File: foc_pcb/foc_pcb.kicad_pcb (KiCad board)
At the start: 2 copper layers, 114.3 x 128.3 mm, 70 parts, among them IC1 AS5600-ASOT, J1 Conn_01x03, J10 Conn_02x03_Top_Bottom, J11 Conn_01x03, J12 10118193-0001LF, J2 Conn_01x03, J3 Conn_01x03, J4 Conn_01x04, J5 XT60PW-M, J6 XT60PW-M, J7 Conn_01x02, J8 Conn_01x02, J9 Conn_01x02, SW1 SW_Push, U1 DRV8313PWPR, U2 ATMEGA328P-AU, U3 BSS138-7-F, U4 BSS138-7-F, U5 CH340C, Y1 ABM3-16MHZ

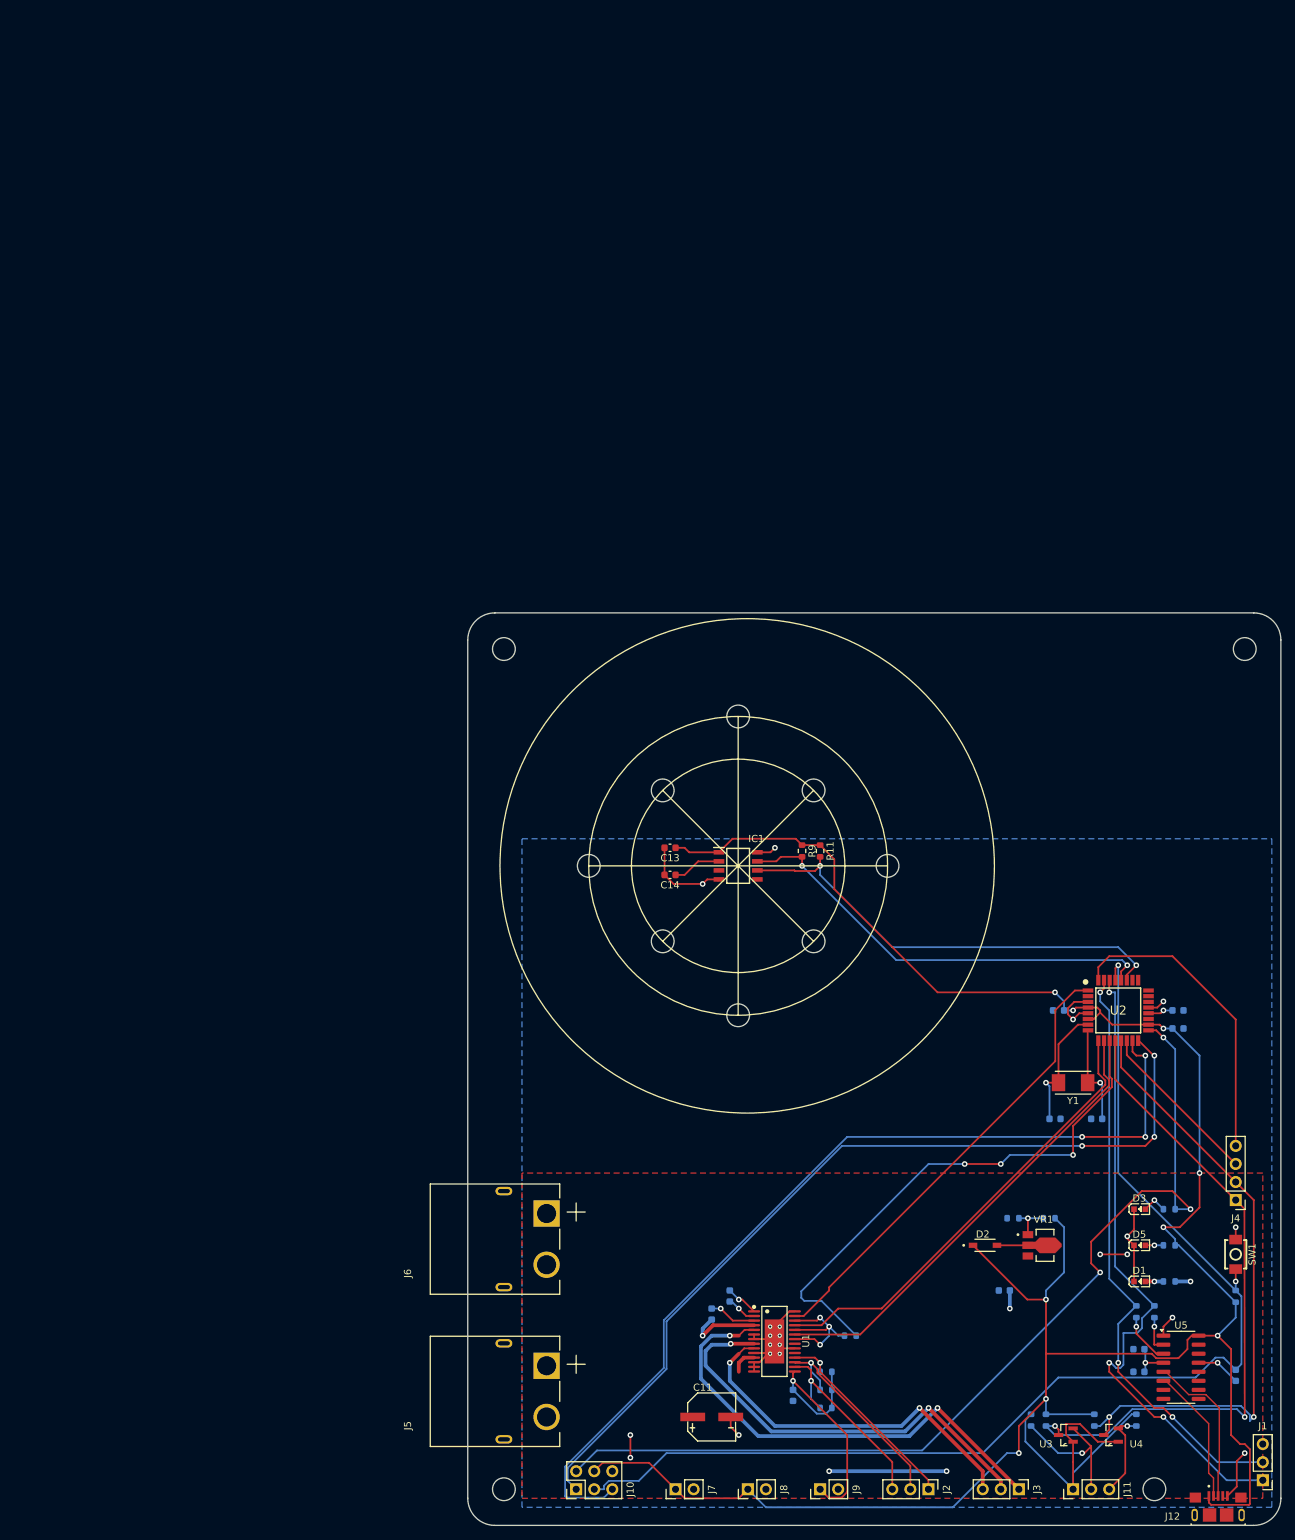
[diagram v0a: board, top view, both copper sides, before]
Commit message: V2 redesign done, needs review
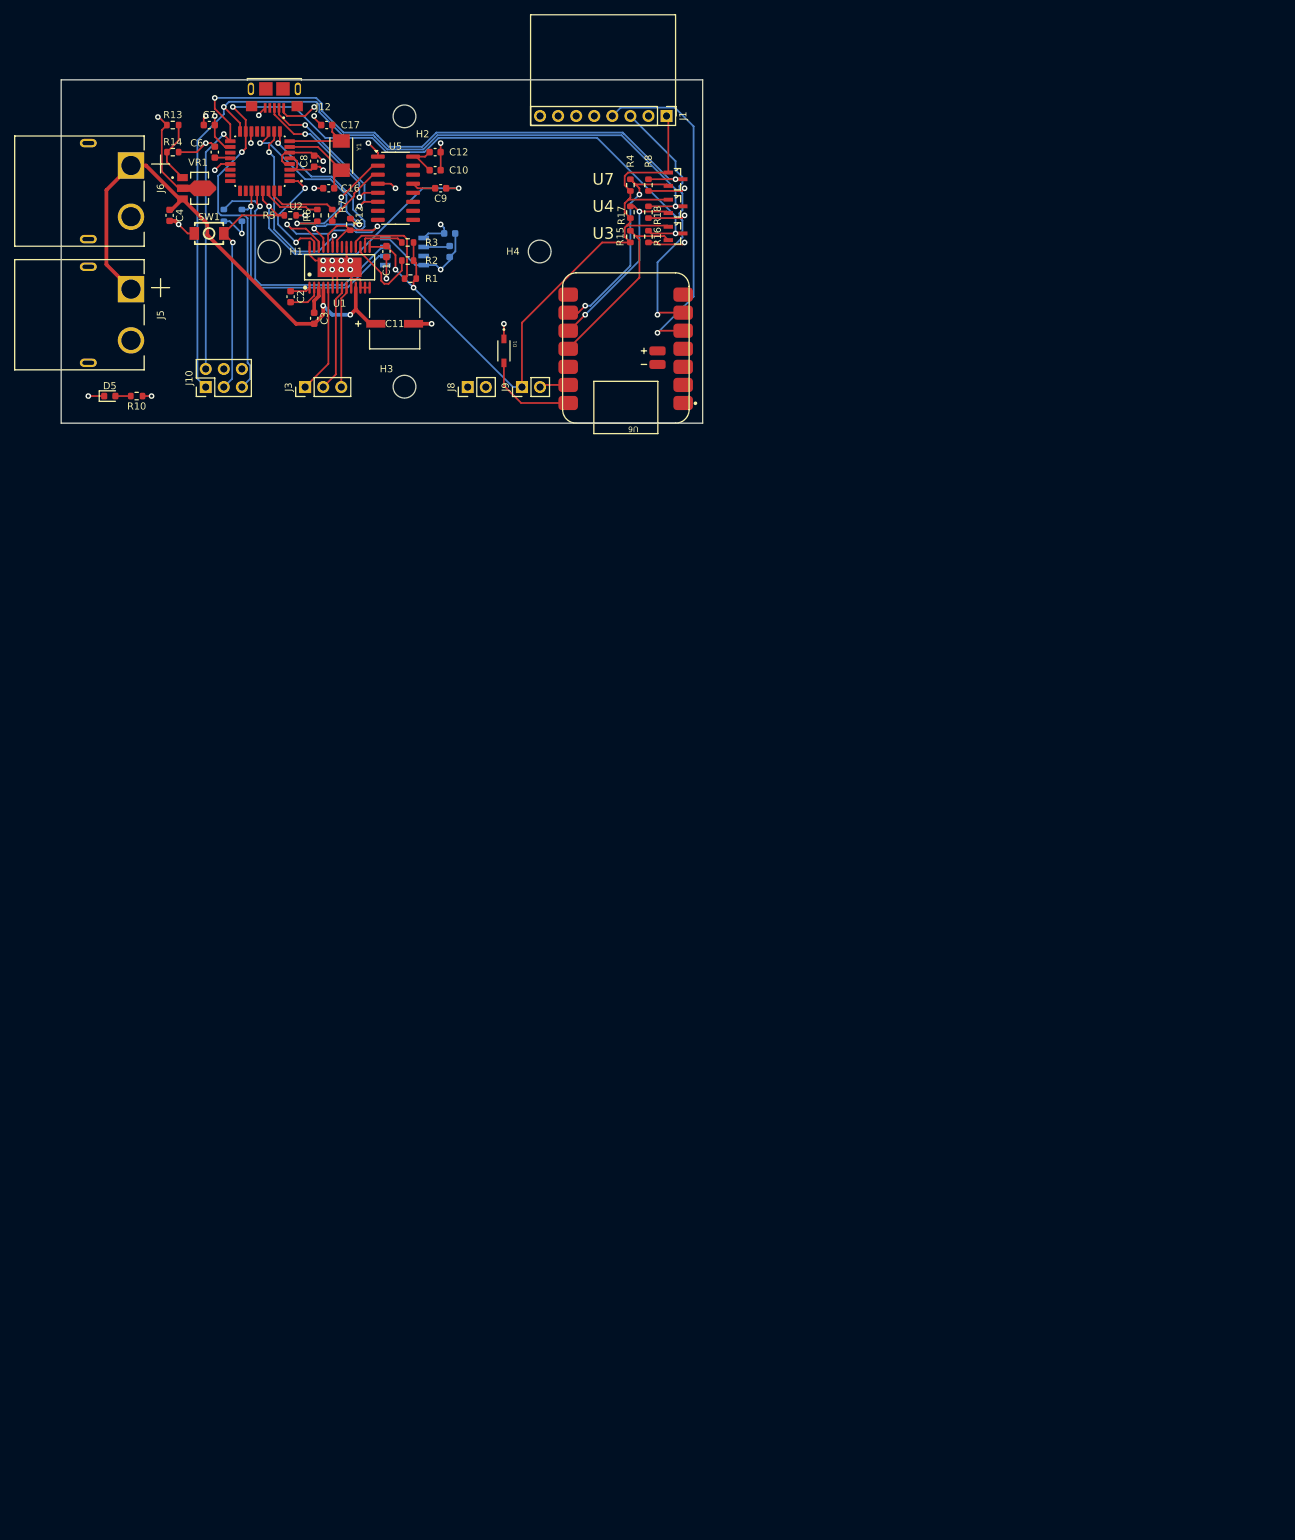
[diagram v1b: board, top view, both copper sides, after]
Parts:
- removed D2: 1N5819HW-7-F, 1N5819HW-7-F:SOD3715X145N
- removed D3: LED, KT-0603R:LED0603-RD
- removed H10, H11, H12, H9: boardMount, MountingHole:MountingHole_3.2mm_M3
- removed H5, H6, H7, H8: motorMount, MountingHole:MountingHole_3.2mm_M3
- removed J11, J2: Conn_01x03, Connector_PinHeader_2.54mm:PinHeader_1x03_P2.54mm_Vertical
- removed J4: Conn_01x04, Connector_PinHeader_2.54mm:PinHeader_1x04_P2.54mm_Vertical
- removed J7: Conn_01x02, Connector_PinHeader_2.54mm:PinHeader_1x02_P2.54mm_Vertical
- added U6: ~, XIAO-ESP32S3:MOUDLE14P-SMD-2.54-21X17.8MM, F.Cu at (287.7, 126.4)
- added U7: BSS138-7-F, BSS138-7-F:SOT95P240X110-3N, F.Cu at (285.8, 113.0)
- C1, C10, C12, C16, C17, C2, C3, C4, C6, C7, C8, C9, R1, R10, R12, R13, R14, R15, R16, R17, R18, R2, R3, R5, R6, R7: moved to F.Cu
- C11: value VT1V101M-CRE77 -> UWT1V101MCL1GS; footprint VT1V101M-CRE77:CAP-SMD_BD6.3-L6.6-W6.6-FD -> UWT1V101MCL1GS:PCAP_6.3x7.7-ELECT_NCA-L
- C13, C14, IC1, R11, R9: moved to B.Cu
- D1: value 19-213/Y2C-CQ2R2L/3T(CY) -> 1N5819HW-7-F; footprint simpleFOC_led:LED0603-RD-YELLOW -> 1N5819HW-7-F:SOD3715X145N
- D5: footprint KT-0603R:LED0603-RD -> LED_SMD:LED_0603_1608Metric
- J1: value Conn_01x03 -> MPU6050; footprint Connector_PinHeader_2.54mm:PinHeader_1x03_P2.54mm_Vertical -> Connector_PinHeader_2.54mm:PinHeader_1x08_P2.54mm_Vertical
- R4, R8: value 1k -> 10k; moved to F.Cu
- U2: footprint ATMEGA328P-AU-NEW:QFP80P900X900X120-32N -> ATMEGA328P-AU:QFP80P900X900X120-32N
- moved J12 240.4 mm to (229.4, 100.3), turned to 180 degrees
- moved J1 209.3 mm to (284.5, 104.1), turned to -90 degrees
- moved SW1 203.5 mm to (220.2, 120.7), turned to 0 degrees
- moved R5 201.9 mm to (231.6, 118.1), turned to 0 degrees
- moved C9 200.8 mm to (252.7, 114.3), turned to 180 degrees
- moved U5 199.2 mm to (246.4, 114.3)
- moved C12 197.9 mm to (252.0, 109.2), turned to 180 degrees
- moved R13 197.0 mm to (215.1, 105.4), turned to 0 degrees
- moved R6 193.9 mm to (235.4, 118.1)
- moved C10 193.0 mm to (252.0, 111.8), turned to 0 degrees
- moved C4 191.3 mm to (214.6, 118.1), turned to -90 degrees
- moved R7 191.1 mm to (237.5, 118.1)
- moved R14 190.8 mm to (215.1, 109.2), turned to 0 degrees
- moved VR1 190.3 mm to (218.4, 114.3)
- moved R10 187.9 mm to (210.0, 143.5)
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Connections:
- net /escl renamed /scl
- net /esda renamed /sda
- net /lvRX renamed /esp_mosi
- net /lvTX renamed /esp_miso
- C10 pad 1: Net-(U5-V3) -> Net-(U5-VCC)
- C12 pad 2: Net-(U5-V3) -> Net-(U5-VCC)
- J1 pad 1: /uRX -> +3.3V
- J1 pad 2: /uTX -> GND
- J1 pad 3: GND -> /esp_scl_1
- R15 pad 1: /3vin -> +3.3V
- R16 pad 2: /aRX1 -> /mosi
- R17 pad 1: /3vin -> +3.3V
- R18 pad 2: /aTX1 -> /miso
- R4 pad 1: VCC -> +3.3V
- R4 pad 2: Net-(D1-A) -> /esp_sck
- R8 pad 1: Net-(D3-A) -> +5V
- U2 pad 12: /aRX1 -> unconnected-(U2-PB0-Pad12)
- U2 pad 13: /aTX1 -> unconnected-(U2-PB1-Pad13)
- U2 pad 14: /aRX2 -> GND
- U2 pad 23: unconnected-(U2-PC0-Pad23) -> /gpio_1
- U2 pad 24: unconnected-(U2-PC1-Pad24) -> /gpio_2
- U2 pad 32: /aTX2 -> unconnected-(U2-PD2-Pad32)
- U3 pad 1: /3vin -> +3.3V
- U3 pad 3: /aRX1 -> /mosi
- U4 pad 1: /3vin -> +3.3V
- U4 pad 3: /aTX1 -> /miso
- U5 pad 16: +5V -> Net-(U5-VCC)
- U5 pad 4: Net-(U5-V3) -> +5V
- VR1 pad 2: Net-(VR1-OUTPUT) -> +5V
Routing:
- net +5V: track 326.2 -> 76.7 mm, vias 9 -> 13
- net /rst: track 168.6 -> 74.3 mm, vias 2 -> 3
- net /aRX1: track 93.7 -> 0.00 mm, vias 2 -> 0
- net /aTX1: track 88.7 -> 0.00 mm, vias 2 -> 0
- net /uRX: track 92.1 -> 8.32 mm, vias 3 -> 0
- net /uTX: track 83.9 -> 9.68 mm, vias 3 -> 0
- net +3.3V: track 38.4 -> 103.4 mm, vias 1 -> 2
- net /out1: track 67.4 -> 15.3 mm, vias 2 -> 0
- net Net-(U2-PD7): track 75.5 -> 23.9 mm, vias 3 -> 2
- net /in1: track 64.7 -> 16.6 mm, vias 0 -> 2
- net /esp_sda_1: track 0.00 -> 47.9 mm, vias 0 -> 1
- net /out2: track 61.3 -> 15.1 mm, vias 2 -> 0
- net /3vin: track 46.2 -> 0.00 mm
- net /aTX2: track 43.3 -> 0.00 mm
- net VCC: track 35.5 -> 76.0 mm, vias 5 -> 2
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- added copper zone on In1.Cu, net +5V
- added copper zone on In2.Cu, net GND
- removed copper zone on B.Cu, net GND
- removed copper zone on F.Cu, net VCC
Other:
- board size 114.3 x 128.3 mm -> 90.2 x 48.3 mm
- copper layers 2 -> 4
